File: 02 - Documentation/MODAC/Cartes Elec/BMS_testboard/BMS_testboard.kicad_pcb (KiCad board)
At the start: 2 copper layers, 20 parts, among them J2 3P Droit 22-11-2032, J3 3P Droit 22-11-2032, Q10 NMOS SQ2348ES-T1_GE3, Q2 PMOS SI2343CDS-T1-GE3, Q3 PMOS SI2343CDS-T1-GE3, Q7 NMOS SQ2348ES-T1_GE3, Q8 NMOS SQ2348ES-T1_GE3, Q9 NMOS SQ2348ES-T1_GE3, U2 74LVC1GU04DRL, U3 74LVC1GU04DRL

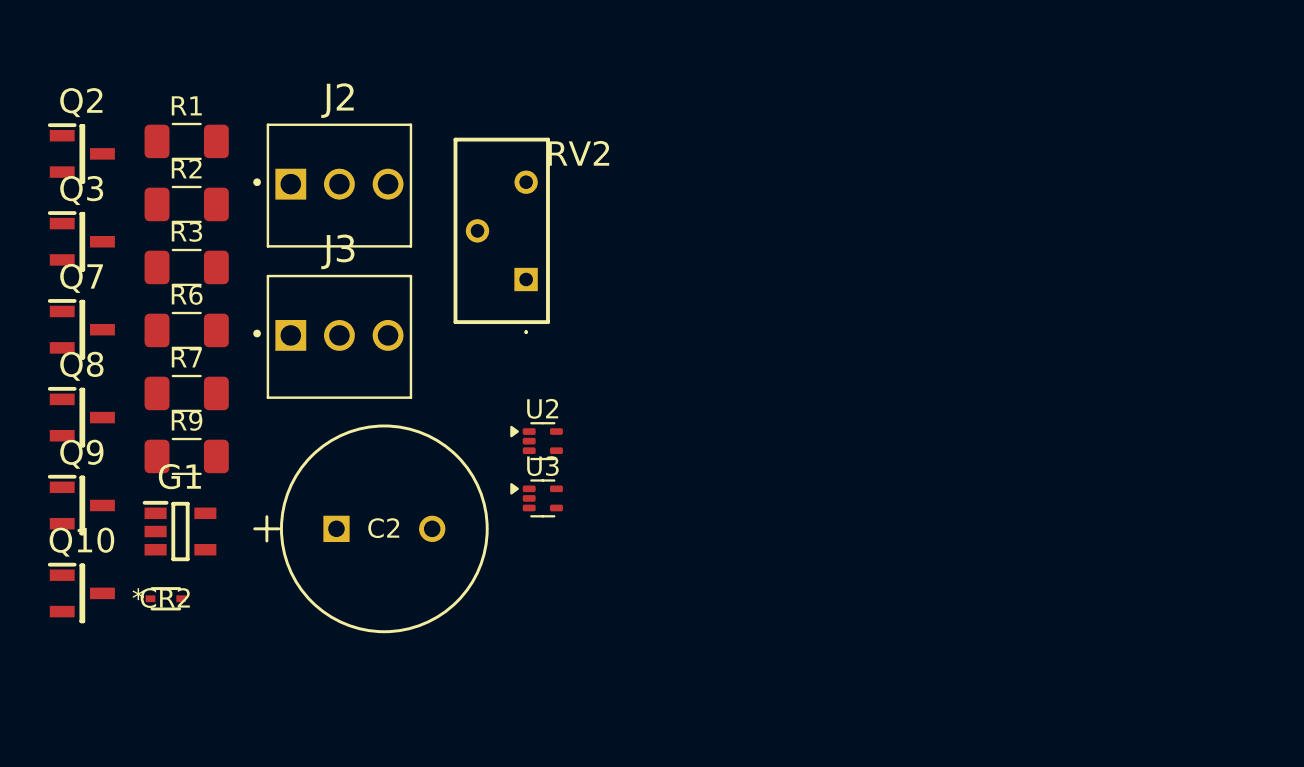
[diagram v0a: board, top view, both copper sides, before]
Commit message: BMS Testboard PCB finito
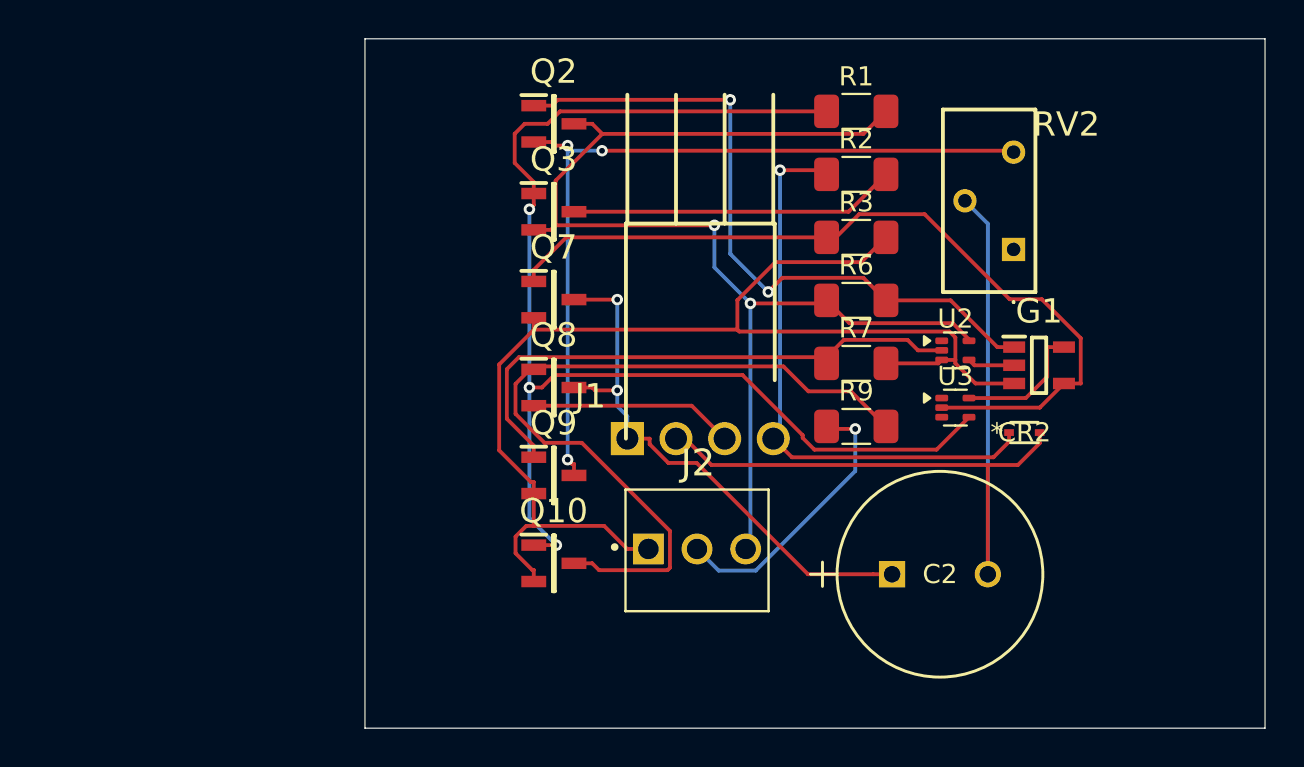
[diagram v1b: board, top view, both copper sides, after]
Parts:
- removed J3: 3P Droit 22-11-2032, EPSA_lib:MOLEX_22-11-2032
- added J1: 4P Angle 171857-4004, EPSA_lib:HDRRA4W66P0X254_1X4_762X818X635P, F.Cu at (77.7, 45.4)
- moved G1 45.7 mm to (99.2, 41.5)
- moved CR2 45.7 mm to (98.4, 45.1)
- moved R1 35.0 mm to (89.7, 28.3)
- moved R2 35.0 mm to (89.7, 31.6)
- moved R3 35.0 mm to (89.7, 34.9)
- moved R6 35.0 mm to (89.7, 38.2)
- moved R7 35.0 mm to (89.7, 41.5)
- moved R9 35.0 mm to (89.7, 44.7)
- moved C2 29.1 mm to (91.5, 52.5)
- moved J2 26.7 mm to (78.8, 51.1)
- moved RV2 25.5 mm to (97.9, 35.5)
- moved Q10 24.7 mm to (73.9, 51.9)
- moved Q2 24.7 mm to (73.9, 28.9)
- moved Q3 24.7 mm to (73.9, 33.5)
- moved Q7 24.7 mm to (73.9, 38.1)
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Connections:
- net C1 renamed C_Down
- CR2 pad 2: Net-(RV2-CW) -> V_cap+
- Q8 pad 2: C2 -> C_Up
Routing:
- net +5V: track 0.00 -> 69.5 mm, vias 0 -> 2
- net A2: track 0.00 -> 66.1 mm, vias 0 -> 3
- net GND: track 0.00 -> 64.3 mm
- net V_cap+: track 0.00 -> 46.3 mm
- net A3: track 0.00 -> 43.2 mm
- net Net-(RV2-CW): track 0.00 -> 42.6 mm, vias 0 -> 3
- net Vgate_enable: track 0.00 -> 40.3 mm
- net A0: track 0.00 -> 35.9 mm, vias 0 -> 2
- net C_Down: track 0.00 -> 30.2 mm, vias 0 -> 1
- net A1: track 0.00 -> 29.1 mm
- net V_cap-: track 0.00 -> 29.0 mm, vias 0 -> 2
- net Net-(Q3-Pad3): track 0.00 -> 17.1 mm
- net +12V: track 0.00 -> 14.6 mm, vias 0 -> 1
- net C_Up: track 0.00 -> 10.7 mm
- net Net-(G1-Pad2): track 0.00 -> 2.47 mm
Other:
- board outline added: 47 x 36 mm
